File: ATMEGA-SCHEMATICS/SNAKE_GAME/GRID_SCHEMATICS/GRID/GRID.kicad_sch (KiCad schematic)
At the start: 42 parts, among them J1 Conn_01x04_Pin, J2 Conn_01x04_Pin

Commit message: .
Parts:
- removed C10, C11, C12, C13, C14, C15, C16, C17, C18, C19, C20, C21, C22, C23, C24, C25, C6, C7, C8, C9: 1uF, Capacitor_SMD:C_0603_1608Metric, symbol Device:C
- removed D1, D10, D11, D13, D14, D15, D16, D2, D21, D22, D23, D24, D25, D3, D4, D5, D6, D7, D8, D9: APA102-2020, LED_SMD:LED-APA102-2020, symbol LED:APA102-2020
- removed J2: Conn_01x04_Pin, Connector_PinSocket_2.54mm:PinSocket_1x04_P2.54mm_Vertical, symbol Connector:Conn_01x04_Pin
- added C137, C138, C139, C140, C141, C142, C143, C144, C145, C146, C147, C148, C149, C150, C151, C152, C153, C154, C155, C156, C157, C158, C159, C160, C161, C162, C163, C164, C165, C166, C167, C168, C169, C170, C171, C172, C173, C174, C175, C176, C177, C178, C179, C180, C181, C182, C183, C184, C185, C186, C187, C188, C189, C190, C191, C192, C193, C194, C195, C196, C197, C198, C199, C200, C201, C202, C203, C204, C205, C206, C207, C208, C209, C210, C211, C212, C213, C214, C215, C216, C217, C218, C219, C220, C221, C222, C223, C224, C225, C226, C227, C228, C229, C230, C231, C232, C233, C234, C235, C236, C237, C238, C239, C240, C241, C242, C243, C244, C245, C246, C247, C248, C249, C250, C251, C252, C253, C254, C255, C256, C257, C258, C259, C26, C260, C261, C262, C263, C264, C265, C266, C267, C268, C269, C270, C271, C272, C273, C274, C275, C276, C277, C278, C279, C280, C281, C282, C283, C284, C42, C43, C44, C45, C46, C47, C48, C49, C50, C51, C52, C53, C54, C55, C56, C57, C58, C59, C60, C61, C62, C63, C64, C65, C66, C67, C68, C69, C70, C71, C72, C73, C74, C75, C76, C77, C78, C79, C80, C81, C82, C83, C84, C85, C86, C87, C88: 1uF, Capacitor_SMD:C_0603_1608Metric, symbol Device:C
- added D100, D101, D102, D103, D104, D105, D106, D107, D108, D109, D110, D111, D112, D113, D114, D115, D116, D117, D118, D119, D120, D121, D122, D123, D124, D125, D126, D127, D128, D129, D130, D131, D132, D133, D134, D135, D136, D137, D138, D139, D140, D141, D142, D143, D144, D145, D146, D147, D148, D149, D150, D151, D152, D153, D154, D155, D156, D157, D158, D159, D160, D161, D162, D163, D164, D165, D166, D167, D168, D169, D17, D170, D171, D172, D173, D174, D175, D176, D177, D178, D179, D18, D180, D181, D182, D183, D184, D185, D186, D187, D188, D189, D19, D190, D191, D192, D193, D194, D195, D196, D197, D198, D199, D20, D200, D201, D202, D203, D204, D205, D206, D207, D208, D209, D210, D211, D212, D213, D214, D218, D222, D226, D26, D27, D28, D29, D30, D31, D32, D33, D34, D35, D36, D37, D38, D39, D40, D41, D42, D43, D44, D45, D46, D47, D48, D49, D50, D51, D52, D53, D54, D55, D56, D57, D58, D59, D60, D61, D62, D63, D64, D65, D66, D67, D68, D69, D70, D71, D72, D73, D74, D75, D76, D77, D78, D79, D80, D81, D82, D83, D84, D85, D86, D87, D88, D89, D90, D91, D92, D93, D94, D95, D96, D97, D98, D99: APA102-2020, LED_SMD:LED-APA102-2020, symbol LED:APA102-2020
- J1: footprint Connector_PinSocket_2.54mm:PinSocket_1x04_P2.54mm_Vertical -> Connector_PinHeader_2.00mm:PinHeader_1x04_P2.00mm_Horizontal
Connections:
- net GND: now also C137.1, C138.1, C139.1, C140.1, C141.1, C142.1, C143.1, C144.1, C145.1, C146.1, C147.1, C148.1, C149.1, C150.1, C151.1, C152.1, C153.1, C154.1, C155.1, C156.1, C157.1, C158.1, C159.1, C160.1, C161.1, C162.1, C163.1, C164.1, C165.1, C166.1, C167.1, C168.1, C169.1, C170.1, C171.1, C172.1, C173.1, C174.1, C175.1, C176.1, C177.1, C178.1, C179.1, C180.1, C181.1, C182.1, C183.1, C184.1, C185.2, C186.2, C187.2, C188.2, C189.2, C190.2, C191.2, C192.2, C193.2, C194.2, C195.2, C196.2, C197.2, C198.2, C199.2, C200.2, C201.2, C202.2, C203.2, C204.2, C205.2, C206.2, C207.2, C208.2, C209.2, C210.2, C211.2, C212.2, C213.2, C214.2, C215.2, C216.2, C217.2, C218.2, C219.2, C220.2, C221.2, C222.2, C223.2, C224.2, C225.2, C226.2, C227.2, C228.2, C229.2, C230.2, C231.2, C232.2, C233.1, C234.1, C235.1, C236.1, C237.1, C238.1, C239.1, C240.1, C241.1, C242.1, C243.1, C244.1, C245.1, C246.1, C247.1, C248.1, C249.1, C250.1, C251.1, C252.1, C253.1, C254.1, C255.1, C256.1, C257.1, C258.1, C259.1, C26.1, C260.1, C261.1, C262.1, C263.1, C264.1, C265.1, C266.1, C267.1, C268.1, C269.1, C270.1, C271.1, C272.1, C273.1, C274.1, C275.1, C276.1, C277.1, C278.1, C279.1, C280.1, C281.1, C282.1, C283.1, C284.1, C42.1, C43.1, C44.1, C45.1, C46.1, C47.1, C48.1, C49.1, C50.1, C51.1, C52.1, C53.1, C54.1, C55.1, C56.1, C57.1, C58.1, C59.1, C60.1, C61.1, C62.1, C63.1, C64.1, C65.1, C66.1, C67.1, C68.1, C69.1, C70.1, C71.1, C72.1, C73.1, C74.1, C75.1, C76.1, C77.1, C78.1, C79.1, C80.1, C81.1, C82.1, C83.1, C84.1, C85.1, C86.1, C87.1, C88.1, D100.6 (GND), D101.6 (GND), D102.6 (GND), D103.6 (GND), D104.6 (GND), D105.6 (GND), D106.6 (GND), D107.6 (GND), D108.6 (GND), D109.6 (GND), D110.6 (GND), D111.6 (GND), D112.6 (GND), D113.6 (GND), D114.6 (GND), D115.6 (GND), D116.6 (GND), D117.6 (GND), D118.6 (GND), D119.6 (GND), D120.6 (GND), D121.6 (GND), D122.6 (GND), D123.6 (GND), D124.6 (GND), D125.6 (GND), D126.6 (GND), D127.6 (GND), D128.6 (GND), D129.6 (GND), D130.6 (GND), D131.6 (GND), D132.6 (GND), D133.6 (GND), D134.6 (GND), D135.6 (GND), D136.6 (GND), D137.6 (GND), D138.6 (GND), D139.6 (GND), D140.6 (GND), D141.6 (GND), D142.6 (GND), D143.6 (GND), D144.6 (GND), D145.6 (GND), D146.6 (GND), D147.6 (GND), D148.6 (GND), D149.6 (GND), D150.6 (GND), D151.6 (GND), D152.6 (GND), D153.6 (GND), D154.6 (GND), D155.6 (GND), D156.6 (GND), D157.6 (GND), D158.6 (GND), D159.6 (GND), D160.6 (GND), D161.6 (GND), D162.6 (GND), D163.6 (GND), D164.6 (GND), D165.6 (GND), D166.6 (GND), D167.6 (GND), D168.6 (GND), D169.6 (GND), D17.6 (GND), D170.6 (GND), D171.6 (GND), D172.6 (GND), D173.6 (GND), D174.6 (GND), D175.6 (GND), D176.6 (GND), D177.6 (GND), D178.6 (GND), D179.6 (GND), D18.6 (GND), D180.6 (GND), D181.6 (GND), D182.6 (GND), D183.6 (GND), D184.6 (GND), D185.6 (GND), D186.6 (GND), D187.6 (GND), D188.6 (GND), D189.6 (GND), D19.6 (GND), D190.6 (GND), D191.6 (GND), D192.6 (GND), D193.6 (GND), D194.6 (GND), D195.6 (GND), D196.6 (GND), D197.6 (GND), D198.6 (GND), D199.6 (GND), D20.6 (GND), D200.6 (GND), D201.6 (GND), D202.6 (GND), D203.6 (GND), D204.6 (GND), D205.6 (GND), D206.6 (GND), D207.6 (GND), D208.6 (GND), D209.6 (GND), D210.6 (GND), D211.6 (GND), D212.6 (GND), D213.6 (GND), D214.6 (GND), D218.6 (GND), D222.6 (GND), D226.6 (GND), D26.6 (GND), D27.6 (GND), D28.6 (GND), D29.6 (GND), D30.6 (GND), D31.6 (GND), D32.6 (GND), D33.6 (GND), D34.6 (GND), D35.6 (GND), D36.6 (GND), D37.6 (GND), D38.6 (GND), D39.6 (GND), D40.6 (GND), D41.6 (GND), D42.6 (GND), D43.6 (GND), D44.6 (GND), D45.6 (GND), D46.6 (GND), D47.6 (GND), D48.6 (GND), D49.6 (GND), D50.6 (GND), D51.6 (GND), D52.6 (GND), D53.6 (GND), D54.6 (GND), D55.6 (GND), D56.6 (GND), D57.6 (GND), D58.6 (GND), D59.6 (GND), D60.6 (GND), D61.6 (GND), D62.6 (GND), D63.6 (GND), D64.6 (GND), D65.6 (GND), D66.6 (GND), D67.6 (GND), D68.6 (GND), D69.6 (GND), D70.6 (GND), D71.6 (GND), D72.6 (GND), D73.6 (GND), D74.6 (GND), D75.6 (GND), D76.6 (GND), D77.6 (GND), D78.6 (GND), D79.6 (GND), D80.6 (GND), D81.6 (GND), D82.6 (GND), D83.6 (GND), D84.6 (GND), D85.6 (GND), D86.6 (GND), D87.6 (GND), D88.6 (GND), D89.6 (GND), D90.6 (GND), D91.6 (GND), D92.6 (GND), D93.6 (GND), D94.6 (GND), D95.6 (GND), D96.6 (GND), D97.6 (GND), D98.6 (GND), D99.6 (GND)
- net VCC: now also C137.2, C138.2, C139.2, C140.2, C141.2, C142.2, C143.2, C144.2, C145.2, C146.2, C147.2, C148.2, C149.2, C150.2, C151.2, C152.2, C153.2, C154.2, C155.2, C156.2, C157.2, C158.2, C159.2, C160.2, C161.2, C162.2, C163.2, C164.2, C165.2, C166.2, C167.2, C168.2, C169.2, C170.2, C171.2, C172.2, C173.2, C174.2, C175.2, C176.2, C177.2, C178.2, C179.2, C180.2, C181.2, C182.2, C183.2, C184.2, C185.1, C186.1, C187.1, C188.1, C189.1, C190.1, C191.1, C192.1, C193.1, C194.1, C195.1, C196.1, C197.1, C198.1, C199.1, C200.1, C201.1, C202.1, C203.1, C204.1, C205.1, C206.1, C207.1, C208.1, C209.1, C210.1, C211.1, C212.1, C213.1, C214.1, C215.1, C216.1, C217.1, C218.1, C219.1, C220.1, C221.1, C222.1, C223.1, C224.1, C225.1, C226.1, C227.1, C228.1, C229.1, C230.1, C231.1, C232.1, C233.2, C234.2, C235.2, C236.2, C237.2, C238.2, C239.2, C240.2, C241.2, C242.2, C243.2, C244.2, C245.2, C246.2, C247.2, C248.2, C249.2, C250.2, C251.2, C252.2, C253.2, C254.2, C255.2, C256.2, C257.2, C258.2, C259.2, C26.2, C260.2, C261.2, C262.2, C263.2, C264.2, C265.2, C266.2, C267.2, C268.2, C269.2, C270.2, C271.2, C272.2, C273.2, C274.2, C275.2, C276.2, C277.2, C278.2, C279.2, C280.2, C281.2, C282.2, C283.2, C284.2, C42.2, C43.2, C44.2, C45.2, C46.2, C47.2, C48.2, C49.2, C50.2, C51.2, C52.2, C53.2, C54.2, C55.2, C56.2, C57.2, C58.2, C59.2, C60.2, C61.2, C62.2, C63.2, C64.2, C65.2, C66.2, C67.2, C68.2, C69.2, C70.2, C71.2, C72.2, C73.2, C74.2, C75.2, C76.2, C77.2, C78.2, C79.2, C80.2, C81.2, C82.2, C83.2, C84.2, C85.2, C86.2, C87.2, C88.2, D100.1 (VDD), D101.1 (VDD), D102.1 (VDD), D103.1 (VDD), D104.1 (VDD), D105.1 (VDD), D106.1 (VDD), D107.1 (VDD), D108.1 (VDD), D109.1 (VDD), D110.1 (VDD), D111.1 (VDD), D112.1 (VDD), D113.1 (VDD), D114.1 (VDD), D115.1 (VDD), D116.1 (VDD), D117.1 (VDD), D118.1 (VDD), D119.1 (VDD), D120.1 (VDD), D121.1 (VDD), D122.1 (VDD), D123.1 (VDD), D124.1 (VDD), D125.1 (VDD), D126.1 (VDD), D127.1 (VDD), D128.1 (VDD), D129.1 (VDD), D130.1 (VDD), D131.1 (VDD), D132.1 (VDD), D133.1 (VDD), D134.1 (VDD), D135.1 (VDD), D136.1 (VDD), D137.1 (VDD), D138.1 (VDD), D139.1 (VDD), D140.1 (VDD), D141.1 (VDD), D142.1 (VDD), D143.1 (VDD), D144.1 (VDD), D145.1 (VDD), D146.1 (VDD), D147.1 (VDD), D148.1 (VDD), D149.1 (VDD), D150.1 (VDD), D151.1 (VDD), D152.1 (VDD), D153.1 (VDD), D154.1 (VDD), D155.1 (VDD), D156.1 (VDD), D157.1 (VDD), D158.1 (VDD), D159.1 (VDD), D160.1 (VDD), D161.1 (VDD), D162.1 (VDD), D163.1 (VDD), D164.1 (VDD), D165.1 (VDD), D166.1 (VDD), D167.1 (VDD), D168.1 (VDD), D169.1 (VDD), D17.1 (VDD), D170.1 (VDD), D171.1 (VDD), D172.1 (VDD), D173.1 (VDD), D174.1 (VDD), D175.1 (VDD), D176.1 (VDD), D177.1 (VDD), D178.1 (VDD), D179.1 (VDD), D18.1 (VDD), D180.1 (VDD), D181.1 (VDD), D182.1 (VDD), D183.1 (VDD), D184.1 (VDD), D185.1 (VDD), D186.1 (VDD), D187.1 (VDD), D188.1 (VDD), D189.1 (VDD), D19.1 (VDD), D190.1 (VDD), D191.1 (VDD), D192.1 (VDD), D193.1 (VDD), D194.1 (VDD), D195.1 (VDD), D196.1 (VDD), D197.1 (VDD), D198.1 (VDD), D199.1 (VDD), D20.1 (VDD), D200.1 (VDD), D201.1 (VDD), D202.1 (VDD), D203.1 (VDD), D204.1 (VDD), D205.1 (VDD), D206.1 (VDD), D207.1 (VDD), D208.1 (VDD), D209.1 (VDD), D210.1 (VDD), D211.1 (VDD), D212.1 (VDD), D213.1 (VDD), D214.1 (VDD), D218.1 (VDD), D222.1 (VDD), D226.1 (VDD), D26.1 (VDD), D27.1 (VDD), D28.1 (VDD), D29.1 (VDD), D30.1 (VDD), D31.1 (VDD), D32.1 (VDD), D33.1 (VDD), D34.1 (VDD), D35.1 (VDD), D36.1 (VDD), D37.1 (VDD), D38.1 (VDD), D39.1 (VDD), D40.1 (VDD), D41.1 (VDD), D42.1 (VDD), D43.1 (VDD), D44.1 (VDD), D45.1 (VDD), D46.1 (VDD), D47.1 (VDD), D48.1 (VDD), D49.1 (VDD), D50.1 (VDD), D51.1 (VDD), D52.1 (VDD), D53.1 (VDD), D54.1 (VDD), D55.1 (VDD), D56.1 (VDD), D57.1 (VDD), D58.1 (VDD), D59.1 (VDD), D60.1 (VDD), D61.1 (VDD), D62.1 (VDD), D63.1 (VDD), D64.1 (VDD), D65.1 (VDD), D66.1 (VDD), D67.1 (VDD), D68.1 (VDD), D69.1 (VDD), D70.1 (VDD), D71.1 (VDD), D72.1 (VDD), D73.1 (VDD), D74.1 (VDD), D75.1 (VDD), D76.1 (VDD), D77.1 (VDD), D78.1 (VDD), D79.1 (VDD), D80.1 (VDD), D81.1 (VDD), D82.1 (VDD), D83.1 (VDD), D84.1 (VDD), D85.1 (VDD), D86.1 (VDD), D87.1 (VDD), D88.1 (VDD), D89.1 (VDD), D90.1 (VDD), D91.1 (VDD), D92.1 (VDD), D93.1 (VDD), D94.1 (VDD), D95.1 (VDD), D96.1 (VDD), D97.1 (VDD), D98.1 (VDD), D99.1 (VDD)
- net at J1.1 (Pin_1): now also D17.4 (SDI)
- net at J1.2 (Pin_2): now also D17.5 (CKI)
- new net: D20.2 (CKO), D26.5 (CKI)
- new net: D20.3 (SDO), D26.4 (SDI)
- new net: D19.3 (SDO), D20.4 (SDI)
- new net: D19.2 (CKO), D20.5 (CKI)
- new net: D95.2 (CKO), D96.5 (CKI)
- new net: D95.3 (SDO), D96.4 (SDI)
- new net: D94.3 (SDO), D95.4 (SDI)
- new net: D94.2 (CKO), D95.5 (CKI)
- new net: D170.2 (CKO), D172.5 (CKI)
- new net: D170.3 (SDO), D172.4 (SDI)
- new net: D168.3 (SDO), D170.4 (SDI)
- new net: D168.2 (CKO), D170.5 (CKI)
- new net: D146.2 (CKO), D148.5 (CKI)
- new net: D146.3 (SDO), D148.4 (SDI)
- new net: D144.3 (SDO), D146.4 (SDI)
- new net: D144.2 (CKO), D146.5 (CKI)
- new net: D145.5 (CKI), D147.2 (CKO)
- new net: D145.4 (SDI), D147.3 (SDO)
- new net: D147.4 (SDI), D149.3 (SDO)
- new net: D147.5 (CKI), D149.2 (CKO)
- new net: D141.5 (CKI), D143.2 (CKO)
- new net: D141.4 (SDI), D143.3 (SDO)
- new net: D143.4 (SDI), D145.3 (SDO)
- new net: D143.5 (CKI), D145.2 (CKO)
- new net: D75.2 (CKO), D76.5 (CKI)
- new net: D75.3 (SDO), D76.4 (SDI)
- new net: D74.3 (SDO), D75.4 (SDI)
- new net: D74.2 (CKO), D75.5 (CKI)
- new net: D198.2 (CKO), D200.5 (CKI)
- new net: D198.3 (SDO), D200.4 (SDI)
- new net: D196.3 (SDO), D198.4 (SDI)
- new net: D196.2 (CKO), D198.5 (CKI)
- new net: D159.5 (CKI), D161.2 (CKO)
- new net: D159.4 (SDI), D161.3 (SDO)
- new net: D161.4 (SDI), D163.3 (SDO)
- new net: D161.5 (CKI), D163.2 (CKO)
- new net: D176.2 (CKO), D178.5 (CKI)
- new net: D176.3 (SDO), D178.4 (SDI)
- new net: D174.3 (SDO), D176.4 (SDI)
- new net: D174.2 (CKO), D176.5 (CKI)
- new net: D119.2 (CKO), D214.5 (CKI)
- new net: D119.3 (SDO), D214.4 (SDI)
- new net: D119.4 (SDI), D121.3 (SDO)
- new net: D119.5 (CKI), D121.2 (CKO)
- new net: D165.5 (CKI), D167.2 (CKO)
- new net: D165.4 (SDI), D167.3 (SDO)
- new net: D167.4 (SDI), D169.3 (SDO)
- new net: D167.5 (CKI), D169.2 (CKO)
- new net: D98.2 (CKO), D99.5 (CKI)
- new net: D98.3 (SDO), D99.4 (SDI)
- new net: D97.3 (SDO), D98.4 (SDI)
- new net: D97.2 (CKO), D98.5 (CKI)
- new net: D172.2 (CKO), D174.5 (CKI)
- new net: D172.3 (SDO), D174.4 (SDI)
- new net: D115.2 (CKO), D116.5 (CKI)
- new net: D115.3 (SDO), D116.4 (SDI)
- new net: D114.3 (SDO), D115.4 (SDI)
- new net: D114.2 (CKO), D115.5 (CKI)
- new net: D49.2 (CKO), D50.5 (CKI)
- new net: D49.3 (SDO), D50.4 (SDI)
- new net: D48.3 (SDO), D49.4 (SDI)
- new net: D48.2 (CKO), D49.5 (CKI)
- new net: D42.2 (CKO), D43.5 (CKI)
- new net: D42.3 (SDO), D43.4 (SDI)
- new net: D41.3 (SDO), D42.4 (SDI)
- new net: D41.2 (CKO), D42.5 (CKI)
- new net: D58.2 (CKO), D59.5 (CKI)
- new net: D58.3 (SDO), D59.4 (SDI)
- new net: D57.3 (SDO), D58.4 (SDI)
- new net: D57.2 (CKO), D58.5 (CKI)
- new net: D38.2 (CKO), D39.5 (CKI)
- new net: D38.3 (SDO), D39.4 (SDI)
- new net: D37.3 (SDO), D38.4 (SDI)
- new net: D37.2 (CKO), D38.5 (CKI)
- new net: D222.3 (SDO), D226.4 (SDI)
- new net: D222.2 (CKO), D226.5 (CKI)
- new net: D86.2 (CKO), D87.5 (CKI)
- new net: D86.3 (SDO), D87.4 (SDI)
- new net: D85.3 (SDO), D86.4 (SDI)
- new net: D85.2 (CKO), D86.5 (CKI)
- new net: D205.5 (CKI), D207.2 (CKO)
- new net: D205.4 (SDI), D207.3 (SDO)
- new net: D207.4 (SDI), D209.3 (SDO)
- new net: D207.5 (CKI), D209.2 (CKO)
- new net: D186.2 (CKO), D188.5 (CKI)
- new net: D186.3 (SDO), D188.4 (SDI)
- new net: D184.3 (SDO), D186.4 (SDI)
- new net: D184.2 (CKO), D186.5 (CKI)
- new net: D180.2 (CKO), D182.5 (CKI)
- new net: D180.3 (SDO), D182.4 (SDI)
- new net: D178.3 (SDO), D180.4 (SDI)
- new net: D178.2 (CKO), D180.5 (CKI)
- new net: D183.5 (CKI), D185.2 (CKO)
- new net: D183.4 (SDI), D185.3 (SDO)
- new net: D185.4 (SDI), D187.3 (SDO)
- new net: D185.5 (CKI), D187.2 (CKO)
- new net: D152.2 (CKO), D154.5 (CKI)
- new net: D152.3 (SDO), D154.4 (SDI)
- new net: D150.3 (SDO), D152.4 (SDI)
- new net: D150.2 (CKO), D152.5 (CKI)
- new net: D60.2 (CKO), D61.5 (CKI)
- new net: D60.3 (SDO), D61.4 (SDI)
- new net: D59.3 (SDO), D60.4 (SDI)
- new net: D59.2 (CKO), D60.5 (CKI)
- new net: D70.2 (CKO), D71.5 (CKI)
- new net: D70.3 (SDO), D71.4 (SDI)
- new net: D69.3 (SDO), D70.4 (SDI)
- new net: D69.2 (CKO), D70.5 (CKI)
- new net: D166.2 (CKO), D168.5 (CKI)
- new net: D166.3 (SDO), D168.4 (SDI)
- new net: D164.3 (SDO), D166.4 (SDI)
- new net: D164.2 (CKO), D166.5 (CKI)
- new net: D173.5 (CKI), D175.2 (CKO)
- new net: D173.4 (SDI), D175.3 (SDO)
- new net: D175.4 (SDI), D177.3 (SDO)
- new net: D175.5 (CKI), D177.2 (CKO)
- new net: D126.2 (CKO), D128.5 (CKI)
- new net: D126.3 (SDO), D128.4 (SDI)
- new net: D124.3 (SDO), D126.4 (SDI)
- new net: D124.2 (CKO), D126.5 (CKI)
- new net: D182.2 (CKO), D184.5 (CKI)
- new net: D182.3 (SDO), D184.4 (SDI)
- new net: D201.5 (CKI), D203.2 (CKO)
- new net: D201.4 (SDI), D203.3 (SDO)
- new net: D203.4 (SDI), D205.3 (SDO)
- new net: D203.5 (CKI), D205.2 (CKO)
- new net: D44.2 (CKO), D45.5 (CKI)
- new net: D44.3 (SDO), D45.4 (SDI)
- new net: D43.3 (SDO), D44.4 (SDI)
- new net: D43.2 (CKO), D44.5 (CKI)
- new net: D84.3 (SDO), D85.4 (SDI)
- new net: D84.2 (CKO), D85.5 (CKI)
- new net: D148.3 (SDO), D150.4 (SDI)
- new net: D148.2 (CKO), D150.5 (CKI)
- new net: D137.5 (CKI), D139.2 (CKO)
- new net: D137.4 (SDI), D139.3 (SDO)
- new net: D139.4 (SDI), D141.3 (SDO)
- new net: D139.5 (CKI), D141.2 (CKO)
- new net: D142.3 (SDO), D144.4 (SDI)
- new net: D142.2 (CKO), D144.5 (CKI)
- new net: D33.2 (CKO), D34.5 (CKI)
- new net: D33.3 (SDO), D34.4 (SDI)
- new net: D32.3 (SDO), D33.4 (SDI)
- new net: D32.2 (CKO), D33.5 (CKI)
- new net: D51.2 (CKO), D52.5 (CKI)
- new net: D51.3 (SDO), D52.4 (SDI)
- new net: D50.3 (SDO), D51.4 (SDI)
- new net: D50.2 (CKO), D51.5 (CKI)
- new net: D202.2 (CKO), D204.5 (CKI)
- new net: D202.3 (SDO), D204.4 (SDI)
- new net: D200.3 (SDO), D202.4 (SDI)
- new net: D200.2 (CKO), D202.5 (CKI)
- new net: D56.2 (CKO), D57.5 (CKI)
- new net: D56.3 (SDO), D57.4 (SDI)
- new net: D55.3 (SDO), D56.4 (SDI)
- new net: D55.2 (CKO), D56.5 (CKI)
- new net: D153.5 (CKI), D155.2 (CKO)
- new net: D153.4 (SDI), D155.3 (SDO)
- new net: D155.4 (SDI), D157.3 (SDO)
- new net: D155.5 (CKI), D157.2 (CKO)
- new net: D90.2 (CKO), D91.5 (CKI)
- new net: D90.3 (SDO), D91.4 (SDI)
- new net: D89.3 (SDO), D90.4 (SDI)
- new net: D89.2 (CKO), D90.5 (CKI)
- new net: D140.3 (SDO), D142.4 (SDI)
- new net: D140.2 (CKO), D142.5 (CKI)
- new net: D138.2 (CKO), D140.5 (CKI)
- new net: D138.3 (SDO), D140.4 (SDI)
- new net: D136.3 (SDO), D138.4 (SDI)
- new net: D136.2 (CKO), D138.5 (CKI)
- new net: D82.2 (CKO), D83.5 (CKI)
- new net: D82.3 (SDO), D83.4 (SDI)
- new net: D81.3 (SDO), D82.4 (SDI)
- new net: D81.2 (CKO), D82.5 (CKI)
- new net: D112.2 (CKO), D113.5 (CKI)
- new net: D112.3 (SDO), D113.4 (SDI)
- new net: D111.3 (SDO), D112.4 (SDI)
- new net: D111.2 (CKO), D112.5 (CKI)
- new net: D179.5 (CKI), D181.2 (CKO)
- new net: D179.4 (SDI), D181.3 (SDO)
- new net: D181.4 (SDI), D183.3 (SDO)
- new net: D181.5 (CKI), D183.2 (CKO)
- new net: D149.4 (SDI), D151.3 (SDO)
- new net: D149.5 (CKI), D151.2 (CKO)
- new net: D157.5 (CKI), D159.2 (CKO)
- new net: D157.4 (SDI), D159.3 (SDO)
- new net: D118.2 (CKO), D120.5 (CKI)
- new net: D118.3 (SDO), D120.4 (SDI)
- new net: D117.3 (SDO), D118.4 (SDI)
- new net: D117.2 (CKO), D118.5 (CKI)
- new net: D156.2 (CKO), D158.5 (CKI)
- new net: D156.3 (SDO), D158.4 (SDI)
- new net: D154.3 (SDO), D156.4 (SDI)
- new net: D154.2 (CKO), D156.5 (CKI)
- new net: D104.2 (CKO), D105.5 (CKI)
- new net: D104.3 (SDO), D105.4 (SDI)
- new net: D103.3 (SDO), D104.4 (SDI)
- new net: D103.2 (CKO), D104.5 (CKI)
- new net: D54.3 (SDO), D55.4 (SDI)
- new net: D54.2 (CKO), D55.5 (CKI)
- new net: D211.5 (CKI), D213.2 (CKO)
- new net: D211.4 (SDI), D213.3 (SDO)
- new net: D212.3 (SDO), D213.4 (SDI)
- new net: D212.2 (CKO), D213.5 (CKI)
- new net: D121.4 (SDI), D123.3 (SDO)
- new net: D121.5 (CKI), D123.2 (CKO)
- new net: D34.2 (CKO), D35.5 (CKI)
- new net: D34.3 (SDO), D35.4 (SDI)
- new net: D83.2 (CKO), D84.5 (CKI)
- new net: D83.3 (SDO), D84.4 (SDI)
- new net: D96.2 (CKO), D97.5 (CKI)
- new net: D96.3 (SDO), D97.4 (SDI)
- new net: D68.2 (CKO), D69.5 (CKI)
- new net: D68.3 (SDO), D69.4 (SDI)
- new net: D67.3 (SDO), D68.4 (SDI)
- new net: D67.2 (CKO), D68.5 (CKI)
- new net: D129.5 (CKI), D131.2 (CKO)
- new net: D129.4 (SDI), D131.3 (SDO)
- new net: D131.4 (SDI), D133.3 (SDO)
- new net: D131.5 (CKI), D133.2 (CKO)
- new net: D65.2 (CKO), D66.5 (CKI)
- new net: D65.3 (SDO), D66.4 (SDI)
- new net: D64.3 (SDO), D65.4 (SDI)
- new net: D64.2 (CKO), D65.5 (CKI)
- new net: D218.2 (CKO), D222.5 (CKI)
- new net: D218.3 (SDO), D222.4 (SDI)
- new net: D214.3 (SDO), D218.4 (SDI)
- new net: D214.2 (CKO), D218.5 (CKI)
- new net: D151.5 (CKI), D153.2 (CKO)
- new net: D151.4 (SDI), D153.3 (SDO)
- new net: D36.3 (SDO), D37.4 (SDI)
- new net: D36.2 (CKO), D37.5 (CKI)
- new net: D18.2 (CKO), D19.5 (CKI)
- new net: D18.3 (SDO), D19.4 (SDI)
- new net: D17.3 (SDO), D18.4 (SDI)
- new net: D17.2 (CKO), D18.5 (CKI)
- new net: D79.2 (CKO), D80.5 (CKI)
- new net: D79.3 (SDO), D80.4 (SDI)
- new net: D78.3 (SDO), D79.4 (SDI)
- new net: D78.2 (CKO), D79.5 (CKI)
- new net: D73.2 (CKO), D74.5 (CKI)
- new net: D73.3 (SDO), D74.4 (SDI)
- new net: D72.3 (SDO), D73.4 (SDI)
- new net: D72.2 (CKO), D73.5 (CKI)
- new net: D162.2 (CKO), D164.5 (CKI)
- new net: D162.3 (SDO), D164.4 (SDI)
- new net: D160.3 (SDO), D162.4 (SDI)
- new net: D160.2 (CKO), D162.5 (CKI)
- new net: D116.3 (SDO), D117.4 (SDI)
- new net: D116.2 (CKO), D117.5 (CKI)
- new net: D40.2 (CKO), D41.5 (CKI)
- new net: D40.3 (SDO), D41.4 (SDI)
- new net: D39.3 (SDO), D40.4 (SDI)
- new net: D39.2 (CKO), D40.5 (CKI)
- new net: D106.2 (CKO), D107.5 (CKI)
- new net: D106.3 (SDO), D107.4 (SDI)
- new net: D105.3 (SDO), D106.4 (SDI)
- new net: D105.2 (CKO), D106.5 (CKI)
- new net: D107.2 (CKO), D108.5 (CKI)
- new net: D107.3 (SDO), D108.4 (SDI)
- new net: D35.2 (CKO), D36.5 (CKI)
- new net: D35.3 (SDO), D36.4 (SDI)
- new net: D210.2 (CKO), D212.5 (CKI)
- new net: D210.3 (SDO), D212.4 (SDI)
- new net: D208.3 (SDO), D210.4 (SDI)
- new net: D208.2 (CKO), D210.5 (CKI)
- new net: D53.3 (SDO), D54.4 (SDI)
- new net: D53.2 (CKO), D54.5 (CKI)
- new net: D45.2 (CKO), D46.5 (CKI)
- new net: D45.3 (SDO), D46.4 (SDI)
- new net: D171.5 (CKI), D173.2 (CKO)
- new net: D171.4 (SDI), D173.3 (SDO)
- new net: D88.3 (SDO), D89.4 (SDI)
- new net: D88.2 (CKO), D89.5 (CKI)
- new net: D108.2 (CKO), D109.5 (CKI)
- new net: D108.3 (SDO), D109.4 (SDI)
- new net: D76.2 (CKO), D77.5 (CKI)
- new net: D76.3 (SDO), D77.4 (SDI)
- new net: D31.2 (CKO), D32.5 (CKI)
- new net: D31.3 (SDO), D32.4 (SDI)
- new net: D30.3 (SDO), D31.4 (SDI)
- new net: D30.2 (CKO), D31.5 (CKI)
- new net: D158.3 (SDO), D160.4 (SDI)
- new net: D158.2 (CKO), D160.5 (CKI)
- new net: D52.2 (CKO), D53.5 (CKI)
- new net: D52.3 (SDO), D53.4 (SDI)
- new net: D122.2 (CKO), D124.5 (CKI)
- new net: D122.3 (SDO), D124.4 (SDI)
- new net: D120.3 (SDO), D122.4 (SDI)
- new net: D120.2 (CKO), D122.5 (CKI)
- new net: D66.3 (SDO), D67.4 (SDI)
- new net: D66.2 (CKO), D67.5 (CKI)
- new net: D177.4 (SDI), D179.3 (SDO)
- new net: D177.5 (CKI), D179.2 (CKO)
- new net: D169.4 (SDI), D171.3 (SDO)
- new net: D169.5 (CKI), D171.2 (CKO)
- new net: D125.5 (CKI), D127.2 (CKO)
- new net: D125.4 (SDI), D127.3 (SDO)
- new net: D127.4 (SDI), D129.3 (SDO)
- new net: D127.5 (CKI), D129.2 (CKO)
- new net: D28.2 (CKO), D29.5 (CKI)
- new net: D28.3 (SDO), D29.4 (SDI)
- new net: D27.3 (SDO), D28.4 (SDI)
- new net: D27.2 (CKO), D28.5 (CKI)
- new net: D102.2 (CKO), D103.5 (CKI)
- new net: D102.3 (SDO), D103.4 (SDI)
- new net: D101.3 (SDO), D102.4 (SDI)
- new net: D101.2 (CKO), D102.5 (CKI)
- new net: D134.2 (CKO), D136.5 (CKI)
- new net: D134.3 (SDO), D136.4 (SDI)
- new net: D132.3 (SDO), D134.4 (SDI)
- new net: D132.2 (CKO), D134.5 (CKI)
- new net: D204.2 (CKO), D206.5 (CKI)
- new net: D204.3 (SDO), D206.4 (SDI)
- new net: D194.2 (CKO), D196.5 (CKI)
- new net: D194.3 (SDO), D196.4 (SDI)
- new net: D192.3 (SDO), D194.4 (SDI)
- new net: D192.2 (CKO), D194.5 (CKI)
- new net: D187.4 (SDI), D189.3 (SDO)
- new net: D187.5 (CKI), D189.2 (CKO)
- new net: D110.2 (CKO), D111.5 (CKI)
- new net: D110.3 (SDO), D111.4 (SDI)
- new net: D109.3 (SDO), D110.4 (SDI)
- new net: D109.2 (CKO), D110.5 (CKI)
- new net: D130.3 (SDO), D132.4 (SDI)
- new net: D130.2 (CKO), D132.5 (CKI)
- new net: D113.2 (CKO), D114.5 (CKI)
- new net: D113.3 (SDO), D114.4 (SDI)
- new net: D100.3 (SDO), D101.4 (SDI)
- new net: D100.2 (CKO), D101.5 (CKI)
- new net: D71.3 (SDO), D72.4 (SDI)
- new net: D71.2 (CKO), D72.5 (CKI)
- new net: D209.5 (CKI), D211.2 (CKO)
- new net: D209.4 (SDI), D211.3 (SDO)
- new net: D93.3 (SDO), D94.4 (SDI)
- new net: D93.2 (CKO), D94.5 (CKI)
- new net: D26.3 (SDO), D27.4 (SDI)
- new net: D26.2 (CKO), D27.5 (CKI)
- new net: D80.2 (CKO), D81.5 (CKI)
- new net: D80.3 (SDO), D81.4 (SDI)
- new net: D193.5 (CKI), D195.2 (CKO)
- new net: D193.4 (SDI), D195.3 (SDO)
- new net: D195.4 (SDI), D197.3 (SDO)
- new net: D195.5 (CKI), D197.2 (CKO)
- new net: D197.4 (SDI), D199.3 (SDO)
- new net: D197.5 (CKI), D199.2 (CKO)
- new net: D87.3 (SDO), D88.4 (SDI)
- new net: D87.2 (CKO), D88.5 (CKI)
- new net: D206.2 (CKO), D208.5 (CKI)
- new net: D206.3 (SDO), D208.4 (SDI)
- new net: D190.2 (CKO), D192.5 (CKI)
- new net: D190.3 (SDO), D192.4 (SDI)
- new net: D188.3 (SDO), D190.4 (SDI)
- new net: D188.2 (CKO), D190.5 (CKI)
- new net: D199.4 (SDI), D201.3 (SDO)
- new net: D199.5 (CKI), D201.2 (CKO)
- new net: D163.5 (CKI), D165.2 (CKO)
- new net: D163.4 (SDI), D165.3 (SDO)
- new net: D29.2 (CKO), D30.5 (CKI)
- new net: D29.3 (SDO), D30.4 (SDI)
- new net: D92.2 (CKO), D93.5 (CKI)
- new net: D92.3 (SDO), D93.4 (SDI)
- new net: D91.3 (SDO), D92.4 (SDI)
- new net: D91.2 (CKO), D92.5 (CKI)
- new net: D100.5 (CKI), D99.2 (CKO)
- new net: D100.4 (SDI), D99.3 (SDO)
- new net: D133.5 (CKI), D135.2 (CKO)
- new net: D133.4 (SDI), D135.3 (SDO)
- new net: D135.4 (SDI), D137.3 (SDO)
- new net: D135.5 (CKI), D137.2 (CKO)
- new net: D61.2 (CKO), D62.5 (CKI)
- new net: D61.3 (SDO), D62.4 (SDI)
- new net: D123.4 (SDI), D125.3 (SDO)
- new net: D123.5 (CKI), D125.2 (CKO)
- new net: D77.2 (CKO), D78.5 (CKI)
- new net: D77.3 (SDO), D78.4 (SDI)
- new net: D128.2 (CKO), D130.5 (CKI)
- new net: D128.3 (SDO), D130.4 (SDI)
- new net: D63.2 (CKO), D64.5 (CKI)
- new net: D63.3 (SDO), D64.4 (SDI)
- new net: D62.3 (SDO), D63.4 (SDI)
- new net: D62.2 (CKO), D63.5 (CKI)
- new net: D47.2 (CKO), D48.5 (CKI)
- new net: D47.3 (SDO), D48.4 (SDI)
- new net: D46.3 (SDO), D47.4 (SDI)
- new net: D46.2 (CKO), D47.5 (CKI)
- new net: D189.4 (SDI), D191.3 (SDO)
- new net: D189.5 (CKI), D191.2 (CKO)
- new net: D191.4 (SDI), D193.3 (SDO)
- new net: D191.5 (CKI), D193.2 (CKO)

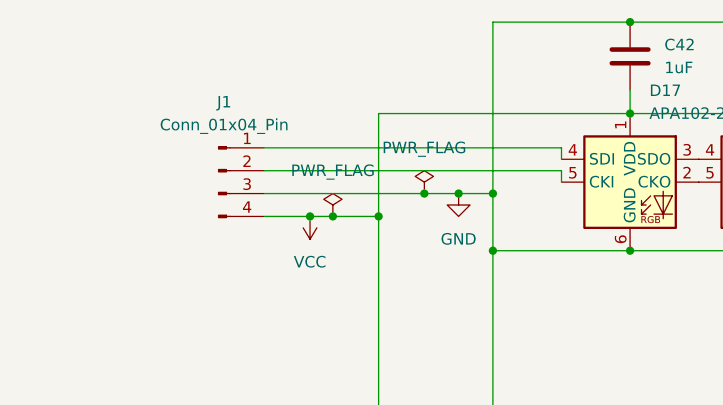
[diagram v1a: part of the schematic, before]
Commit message: ...
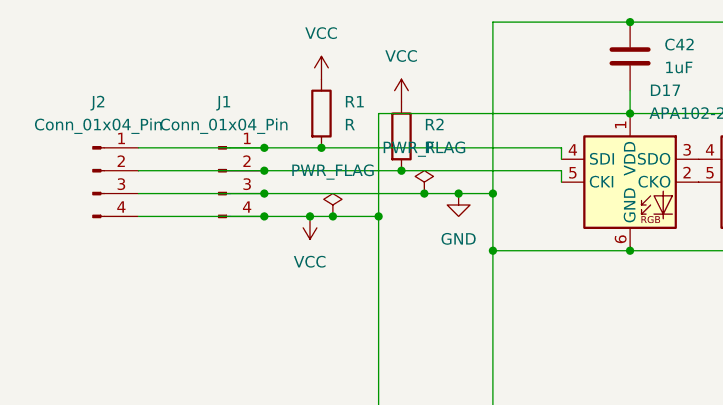
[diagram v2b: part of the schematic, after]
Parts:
- added J2: Conn_01x04_Pin, Connector_PinHeader_2.54mm:PinHeader_1x04_P2.54mm_Vertical, symbol Connector:Conn_01x04_Pin
- added R1, R2: R, Resistor_SMD:R_0402_1005Metric, symbol Device:R
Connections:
- net GND: now also J2.3 (Pin_3)
- net VCC: now also J2.4 (Pin_4), R1.1, R2.1
- net at D17.4 (SDI), J1.1 (Pin_1): now also J2.1 (Pin_1), R1.2
- net at D17.5 (CKI), J1.2 (Pin_2): now also J2.2 (Pin_2), R2.2
